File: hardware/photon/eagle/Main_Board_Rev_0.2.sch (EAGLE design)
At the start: 15 parts, among them IC1 MDC3105LT1, K1 G5LE, U1 RAC02-05SC, X1 MKDSN1,5/3-5,08

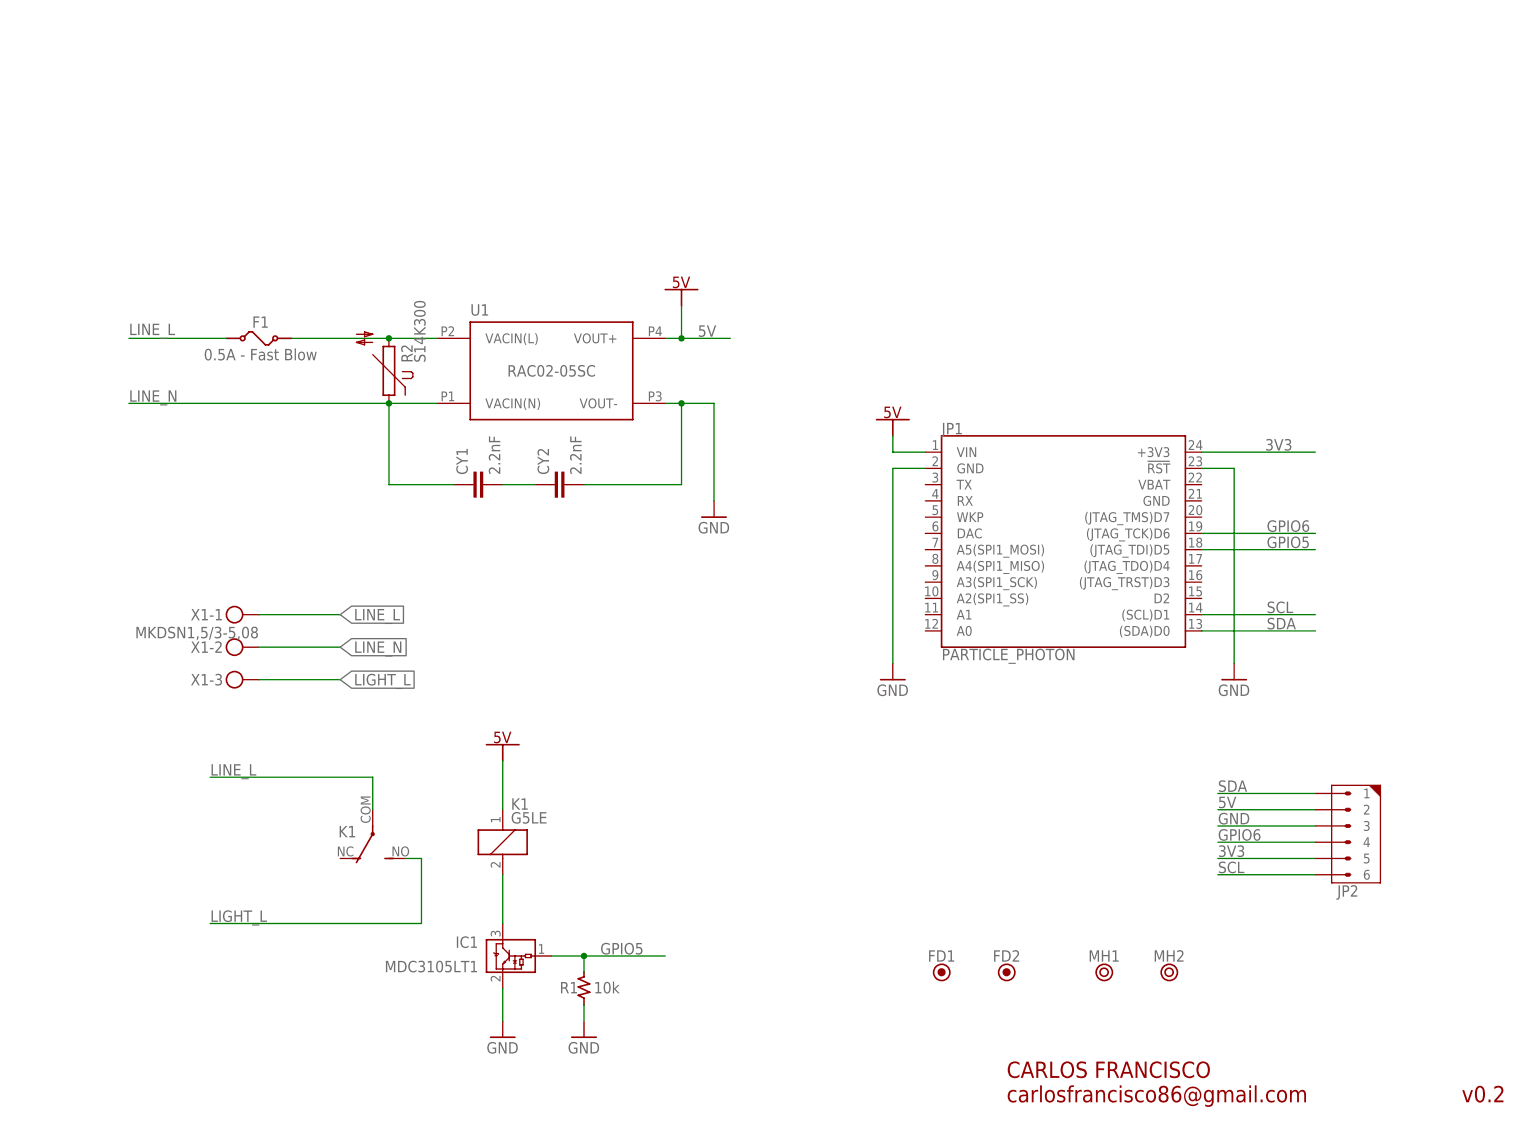
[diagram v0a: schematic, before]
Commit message: Tidy-up
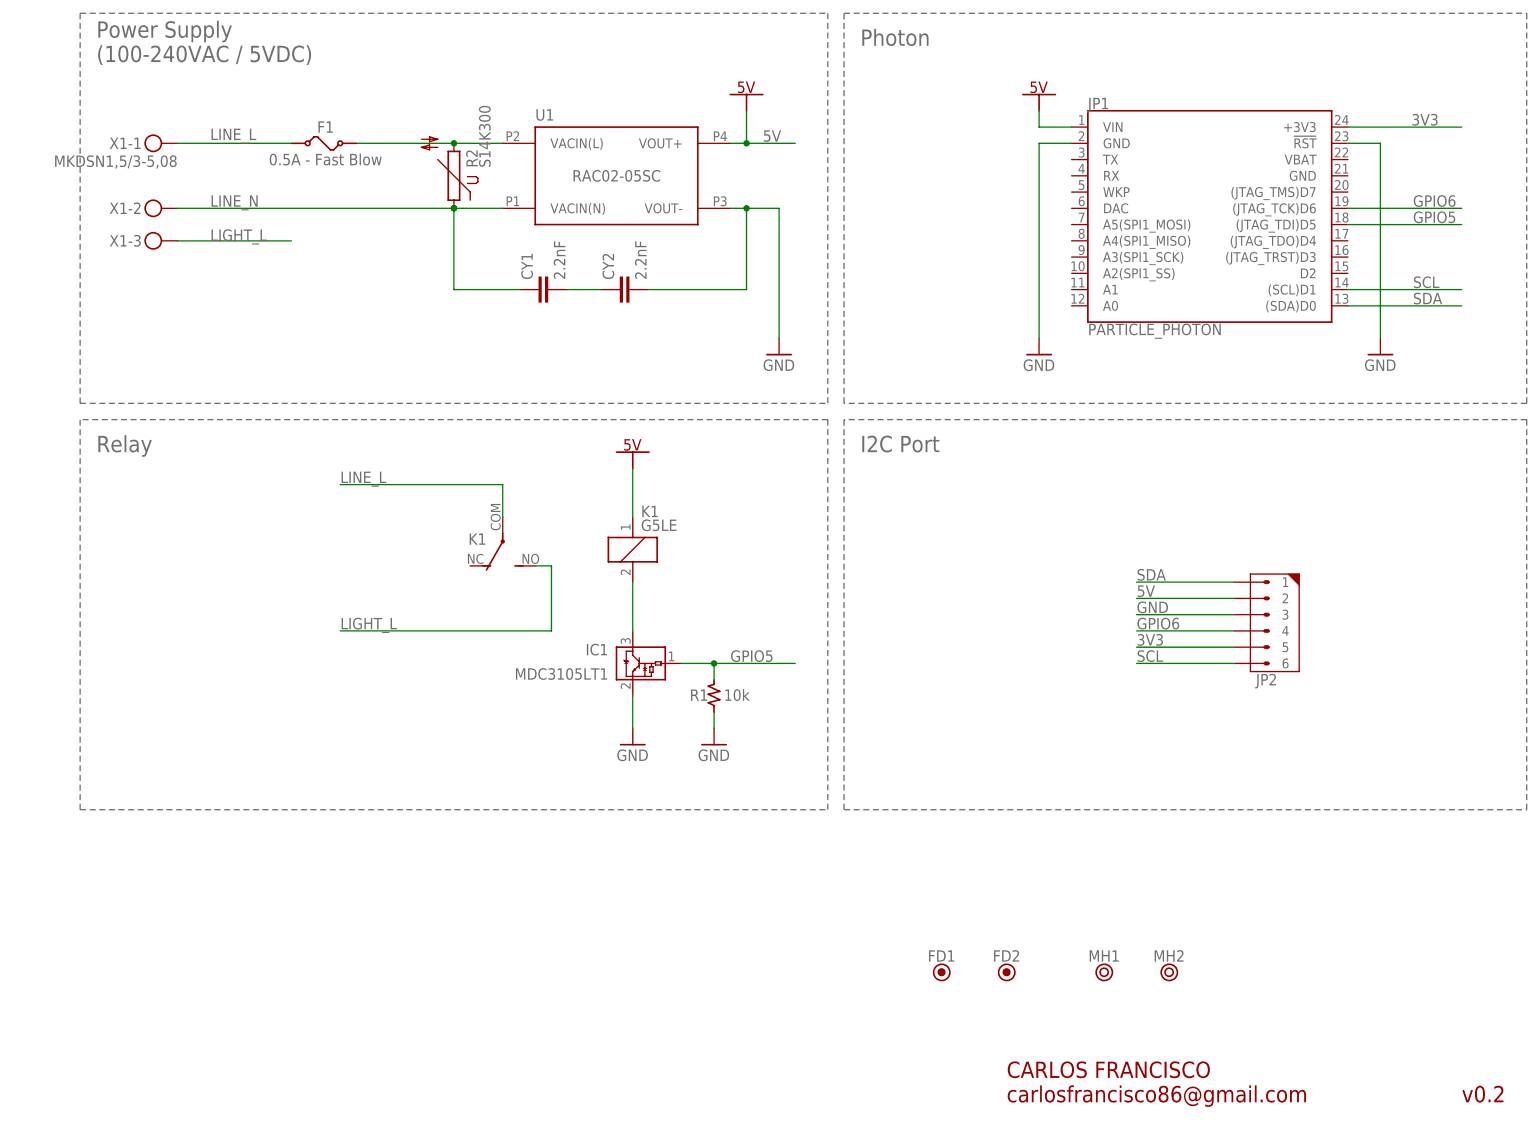
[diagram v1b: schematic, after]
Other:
- note added: "I2C Port"
- note added: "Photon"
- note added: "Power Supply (100-240VAC / 5VDC)"
- note added: "Relay"
- moved on the sheet: CY1, CY2, F1, IC1, JP1, JP2, K1, R1, R2, U1, X1-1, X1-2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
